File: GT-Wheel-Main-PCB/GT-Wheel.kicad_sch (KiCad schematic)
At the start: 69 parts, among them J2 TC2050, J3 0532610471, J4 USB_A, J5 0532610871, J6 0532610871, U1 STM32F303RETx, U2 USB2512B, U3 AP2112K-3.3, X1 8MHz, X2 24MHz

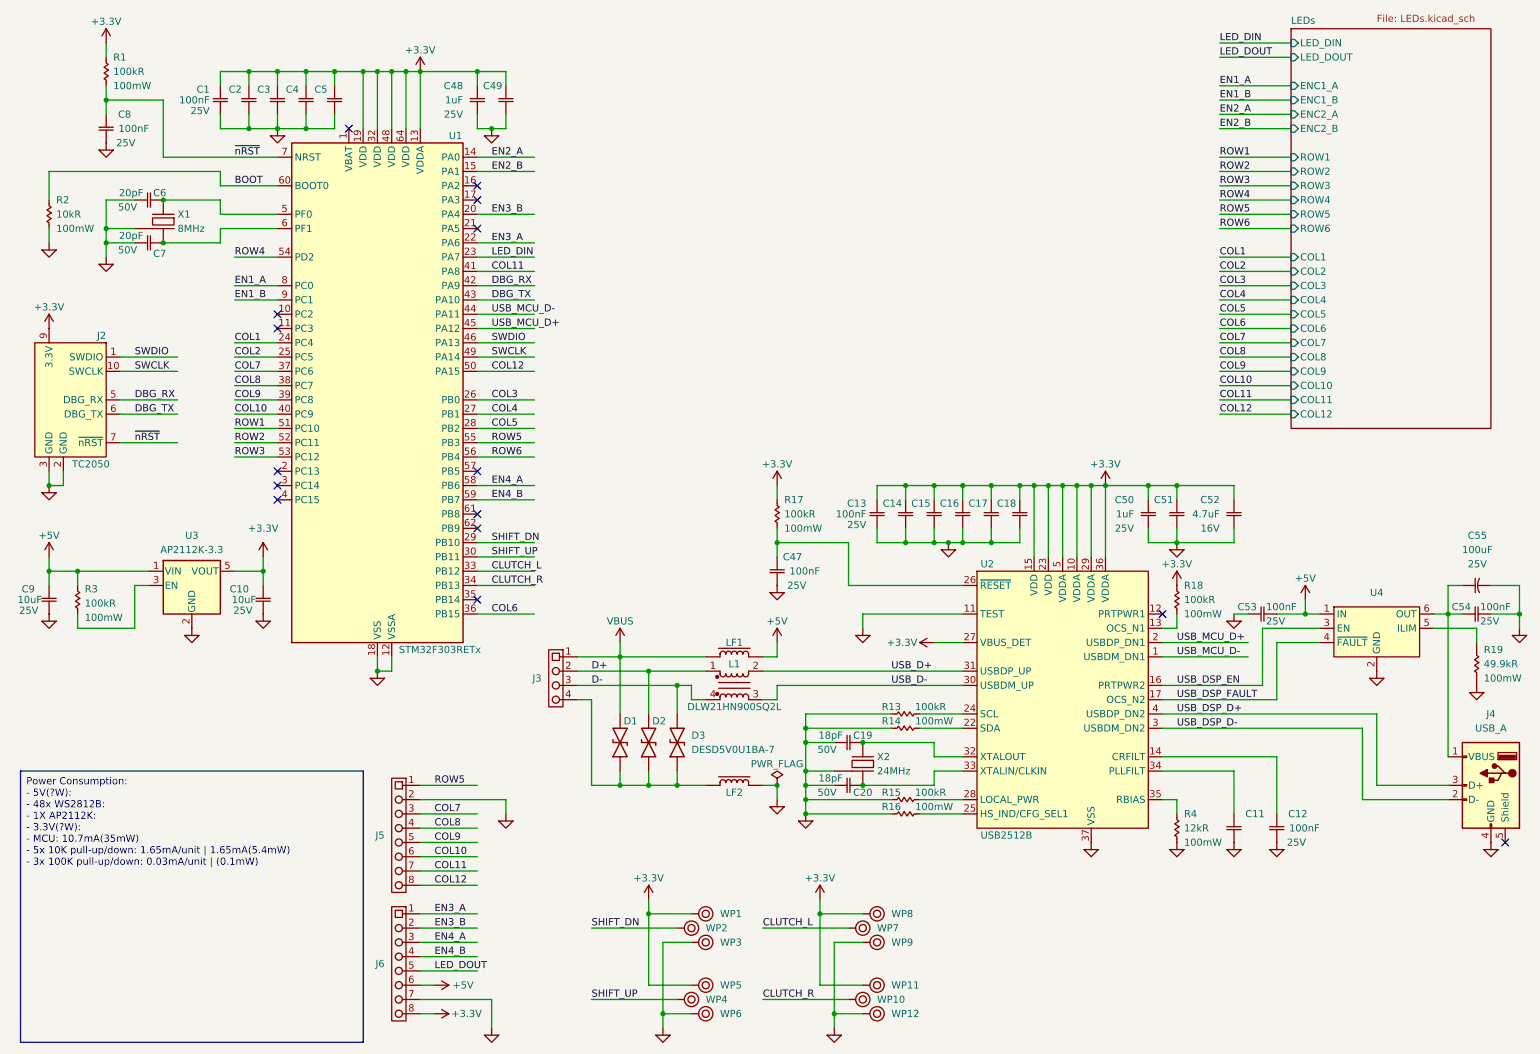
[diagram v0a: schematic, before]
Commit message: updating PCB
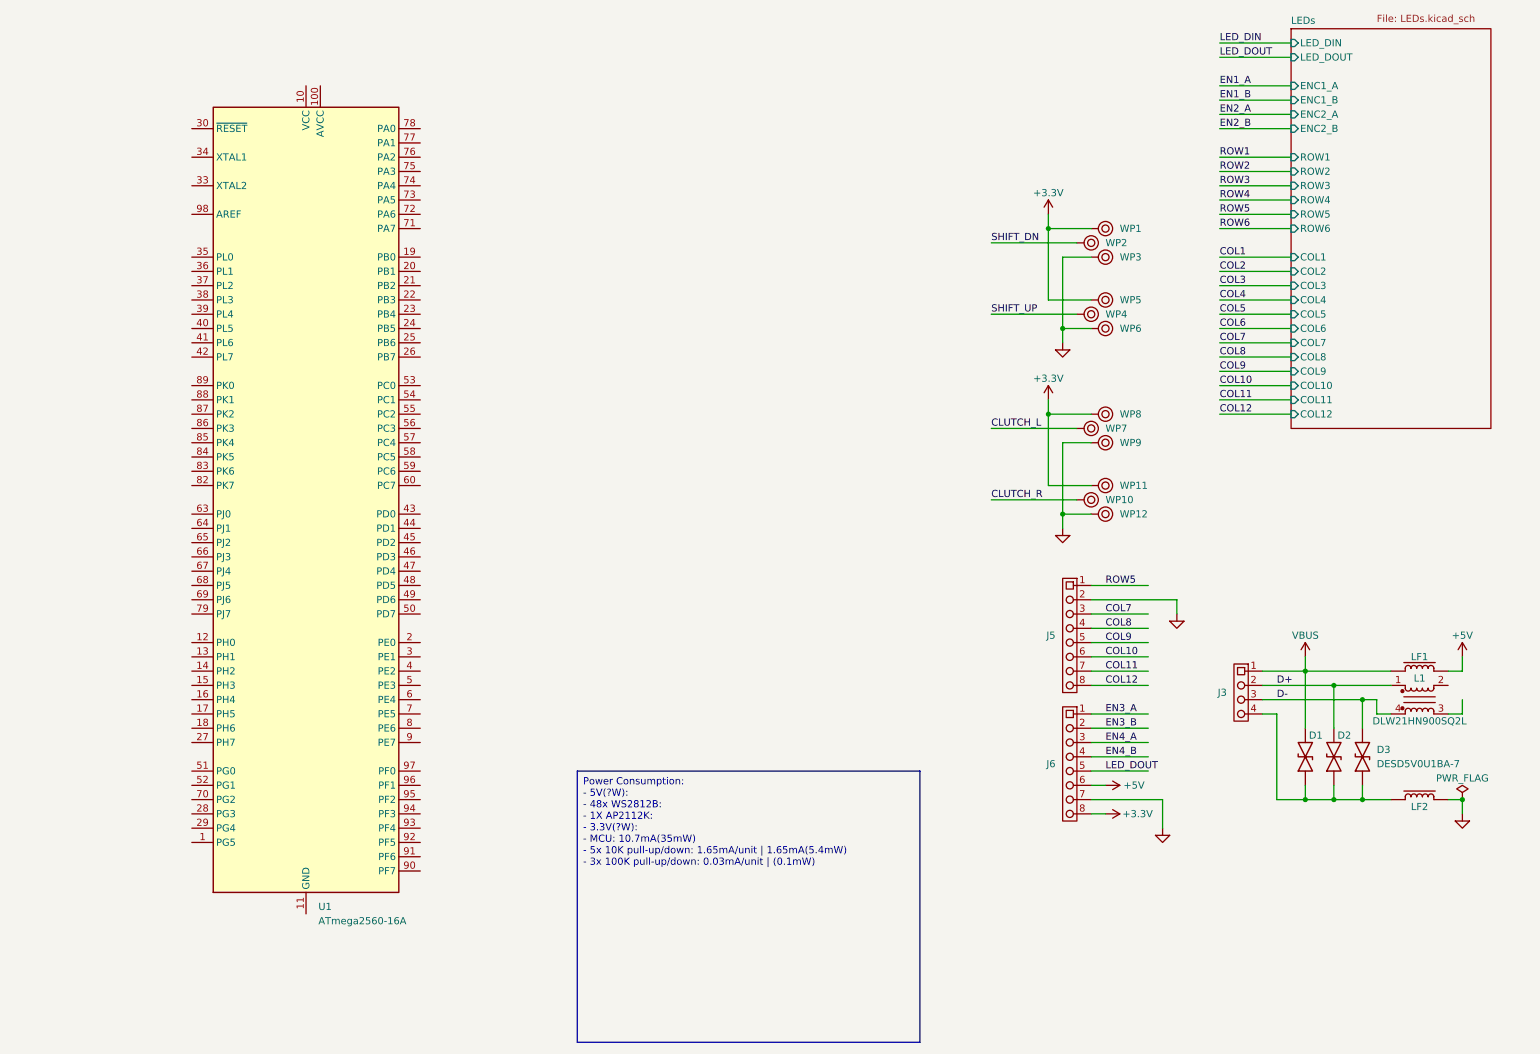
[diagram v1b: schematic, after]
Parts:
- removed C1, C11, C12, C13, C14, C15, C16, C17, C18, C2, C3, C4, C47, C5, C53, C54, C8: 100nF-CER-25V-0402, Capacitor_SMD:C_0402_1005Metric, symbol CAP-SMD-25V:100nF-CER-25V-0402
- removed C10, C9: 10uF-CER-25V-0805, Capacitor_SMD:C_0805_2012Metric, symbol CAP-SMD-25V:10uF-CER-25V-0805
- removed C19, C20: ~, Capacitor_SMD:C_0402_1005Metric, symbol CAP-SMD-50V:18pF-CER-50V-0402
- removed C48, C49, C50, C51: ${SIM.PARAMS}, Capacitor_SMD:C_0805_2012Metric, symbol CAP-SMD-25V:1uF-CER-25V-0805
- removed C52: ${SIM.PARAMS}, Capacitor_SMD:C_0805_2012Metric, symbol CAP-SMD-16V:4.7uF-CER-16V-0805
- removed C55: ${SIM.PARAMS}, Capacitor_SMD:CP_Elec_6.3x5.9, symbol CAP-SMD-25V:100uF-ELEC-50V-RAD6.3Dx6H
- removed C6, C7: ~, Capacitor_SMD:C_0402_1005Metric, symbol CAP-SMD-50V:20pF-CER-50V-0402
- removed J2: TC2050, Connector:Tag-Connect_TC2050-IDC-FP_2x05_P1.27mm_Vertical, symbol CONN-TAG-CONNECT:TC2050
- removed J4: USB_A, CONN-USB:GSB12121RSKHR, symbol Connector:USB_A
- removed R1, R13, R14, R15, R16, R17, R18, R3: 100kR-SMD-100mW-0603, Resistor_SMD:R_0603_1608Metric, symbol RES-SMD-100mW:100kR-SMD-100mW-0603
- removed R19: ${SIM.PARAMS}, Resistor_SMD:R_0603_1608Metric, symbol RES-SMD-100mW:49K9R-SMD-100mW-0603
- removed R2: 10kR-SMD-100mW-0603, Resistor_SMD:R_0603_1608Metric, symbol RES-SMD-100mW:10kR-SMD-100mW-0603
- removed R4: 12kR-SMD-100mW-0603, Resistor_SMD:R_0603_1608Metric, symbol RES-SMD-100mW:12kR-SMD-100mW-0603
- removed U1: STM32F303RETx, Package_QFP:LQFP-64_10x10mm_P0.5mm, symbol MCU_ST_STM32F3:STM32F303RETx
- removed U2: USB2512B, Package_DFN_QFN:QFN-36-1EP_6x6mm_P0.5mm_EP3.7x3.7mm_ThermalVias, symbol IC-SMD-USB-HUB:USB2512B
- removed U3: AP2112K-3.3, Package_TO_SOT_SMD:SOT-23-5, symbol Regulator_Linear:AP2112K-3.3
- removed U4: ~, SOT-SMD:SOT-23-6, symbol IC-SMD-LOAD-SW:AP22653W6-7
- removed X1: 8MHz, Crystal:Crystal_SMD_EuroQuartz_MT-4Pin_3.2x2.5mm, symbol XTAL:XTAL_8MHz_12pF
- removed X2: 24MHz, Crystal:Crystal_SMD_EuroQuartz_MT-4Pin_3.2x2.5mm, symbol XTAL:XTAL_24MHz_6pF
- added U1: ATmega2560-16A, Package_QFP:TQFP-100_14x14mm_P0.5mm, symbol MCU_Microchip_ATmega:ATmega2560-16A
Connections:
- net USB_D+: no longer names the net of L1.2
- net USB_D-: no longer names the net of L1.3
- new net: U1.10 (VCC), U1.31 (VCC), U1.61 (VCC), U1.80 (VCC)
- new net: U1.11 (GND), U1.32 (GND), U1.62 (GND), U1.81 (GND), U1.99 (GND)
- no-connect marks 15 -> 0
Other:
- moved on the sheet: D1, D2, D3, J3, J5, J6, L1, LF1, LF2, WP1, WP10, WP11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
